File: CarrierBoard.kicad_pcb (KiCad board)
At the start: 2 copper layers, 91.4 x 69.1 mm, 5 parts, among them U5 ESP32-S3-DEVKITC-1U-N8R8

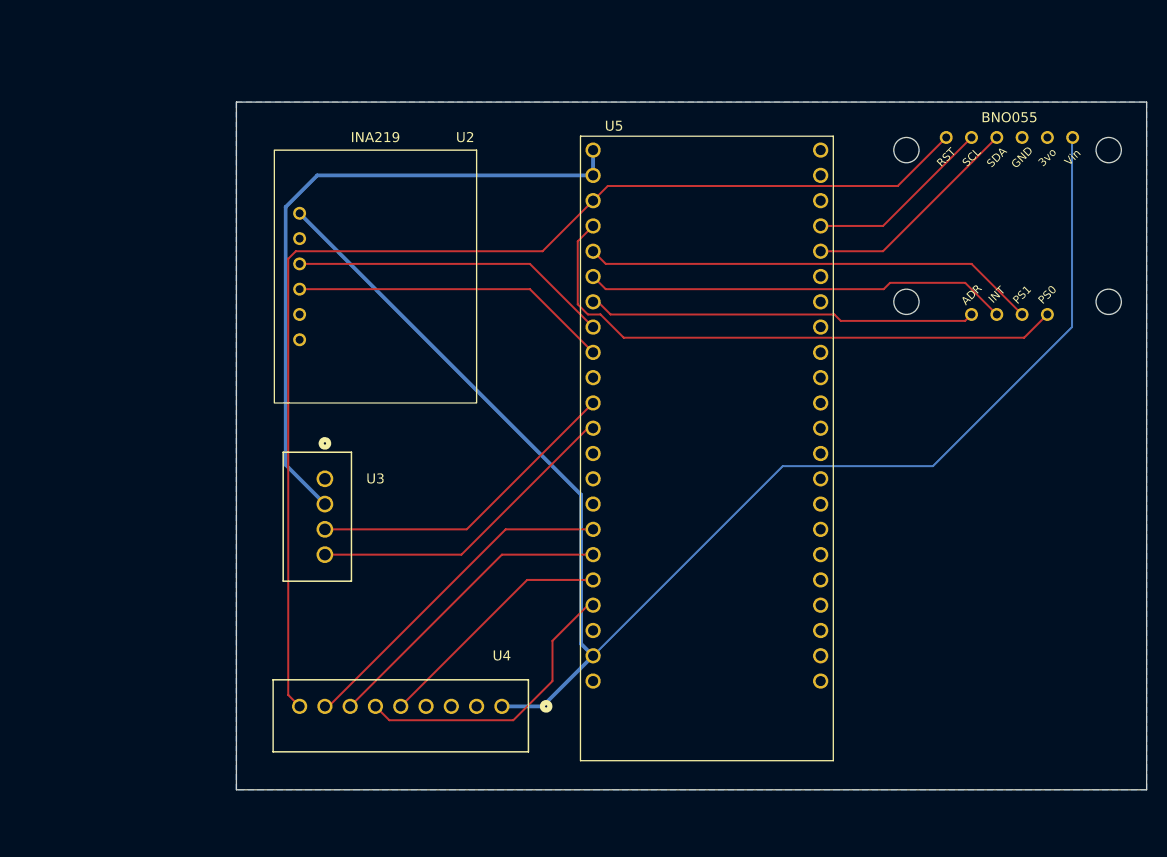
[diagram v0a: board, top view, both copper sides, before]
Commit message: redo board
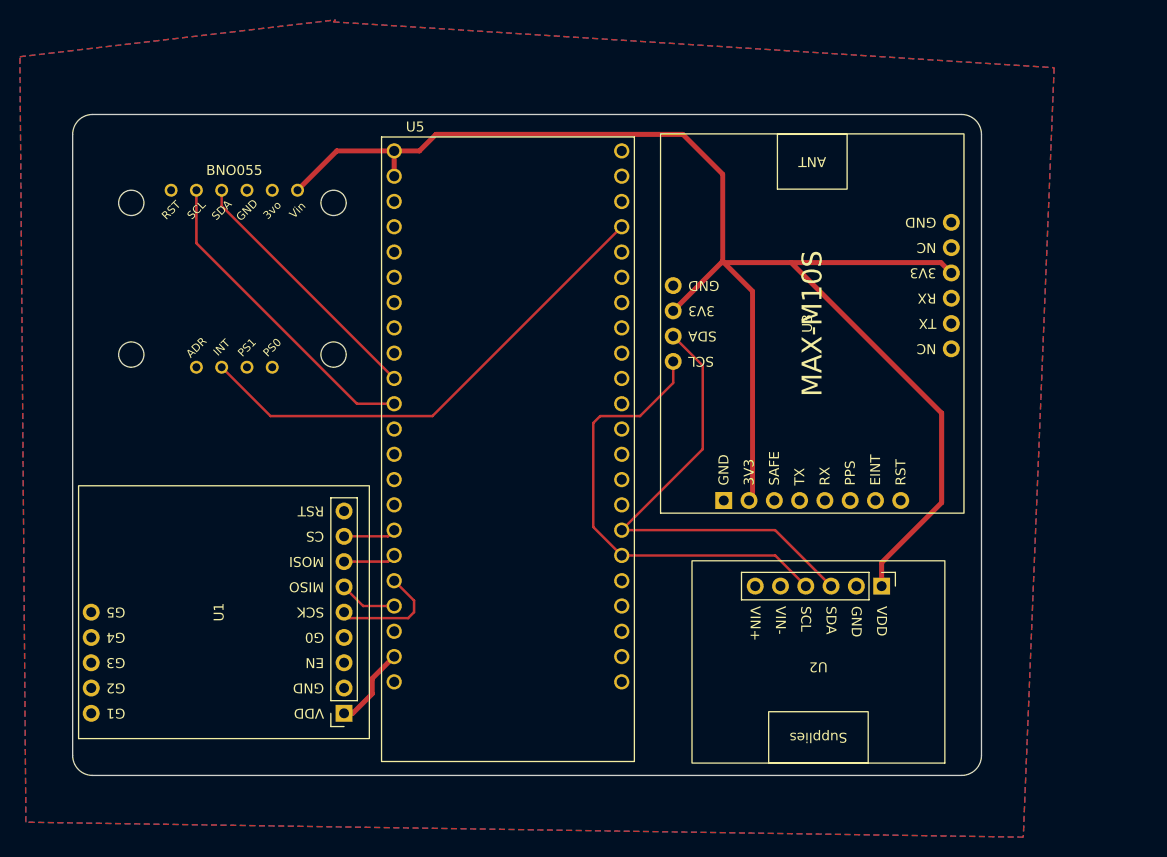
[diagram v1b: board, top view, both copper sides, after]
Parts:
- removed U4: ~, CarrierBoard:TE Connectivity 5-103639-8
- added U6: Adafruit BNO-055, CarrierBoard:Adafruit BNO055, F.Cu at (50.6, 72.6)
- U1: value ~ -> Adafruit RFM95W; footprint CarrierBoard:Adafruit BNO055 -> internalcomponents:Adafruit RFM95W
- U2: value ~ -> Adafruit INA-219; footprint CarrierBoard:Adafruit INA219 -> internalcomponents:INA-219 Adafruit Breakout
- U3: value ~ -> SparkFun MAX-M10S; footprint CarrierBoard:SparkFun MAX-M10S -> internalcomponents:MAX-M10S Sparkfun Breakout
- moved U1 86.8 mm to (55.9, 115.0), turned to 90 degrees
- moved U2 68.9 mm to (115.6, 120.0), turned to 180 degrees
- moved U3 51.4 mm to (115.0, 86.0)
- moved U5 20.0 mm to (84.4, 98.6)
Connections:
- U1 pad 10: Net-(U1-ADR) -> unconnected-(U1-G1-Pad10)
- U1 pad 2: unconnected-(U1-3vo-Pad2) -> GND
- U1 pad 3: GND -> unconnected-(U1-EN-Pad3)
- U1 pad 4: Net-(U1-SDA) -> unconnected-(U1-G0-Pad4)
- U1 pad 5: Net-(U1-SCL) -> /SPI2_SCK
- U1 pad 6: Net-(U1-RST) -> /SPI2_MISO
- U1 pad 7: Net-(U1-PS0) -> /SPI2_MOSI
- U1 pad 8: Net-(U1-PS1) -> /SPI2_CS
- U1 pad 9: Net-(U1-INT) -> unconnected-(U1-RST-Pad9)
- U2 pad 1: +5V -> +3.3V
- U2 pad 3: Net-(U2-SCL) -> /I2C1_SCL
- U2 pad 4: Net-(U2-SDA) -> /I2C1_SDA
- U3 pad 3: Net-(U3-SDA) -> unconnected-(U3-SAFE-Pad3)
- U3 pad 4: Net-(U3-SCL) -> unconnected-(U3-TX-Pad10)
- U5 pad J1_10: unconnected-(U5-GPIO17-PadJ1_10) -> /I2C0_SDA
- U5 pad J1_11: Net-(U3-SDA) -> /I2C0_SCL
- U5 pad J1_12: Net-(U3-SCL) -> unconnected-(U5-GPIO8-PadJ1_12)
- U5 pad J1_16: Net-(U4-CS) -> /SPI2_CS
- U5 pad J1_17: Net-(U4-MOSI) -> /SPI2_MOSI
- U5 pad J1_18: Net-(U4-SCK) -> /SPI2_SCK
- U5 pad J1_19: Net-(U4-MISO) -> /SPI2_MISO
- U5 pad J1_3: Net-(U1-RST) -> unconnected-(U5-RST-PadJ1_3)
- U5 pad J1_4: Net-(U1-PS0) -> unconnected-(U5-GPIO4-PadJ1_4)
- U5 pad J1_5: Net-(U1-PS1) -> unconnected-(U5-GPIO5-PadJ1_5)
- U5 pad J1_6: Net-(U1-INT) -> unconnected-(U5-GPIO6-PadJ1_6)
- U5 pad J1_7: Net-(U1-ADR) -> unconnected-(U5-GPIO7-PadJ1_7)
- U5 pad J1_8: Net-(U2-SCL) -> unconnected-(U5-GPIO15-PadJ1_8)
- U5 pad J1_9: Net-(U2-SDA) -> unconnected-(U5-GPIO16-PadJ1_9)
- U5 pad J3_16: unconnected-(U5-GPIO48-PadJ3_16) -> /I2C1_SCL
- U5 pad J3_17: unconnected-(U5-GPIO47-PadJ3_17) -> /I2C1_SDA
- U5 pad J3_4: Net-(U1-SCL) -> /GYRO_INT
- U5 pad J3_5: Net-(U1-SDA) -> unconnected-(U5-GPIO2-PadJ3_5)
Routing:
- net +5V: track 148.8 -> 8.30 mm
- net Net-(U1-RST): track 116.6 -> 0.00 mm
- net +3.3V: track 66.2 -> 155.2 mm
- net Net-(U1-PS0): track 58.0 -> 0.00 mm
- net /GYRO_INT: track 0.00 -> 50.1 mm
- net /I2C1_SCL: track 0.00 -> 47.4 mm
- net /I2C1_SDA: track 0.00 -> 46.1 mm
- net Net-(U1-PS1): track 45.7 -> 0.00 mm
- net Net-(U1-INT): track 42.7 -> 0.00 mm
- net Net-(U1-ADR): track 39.1 -> 0.00 mm
- net Net-(U4-CS): track 34.3 -> 0.00 mm
- net Net-(U3-SDA): track 32.2 -> 0.00 mm
- net Net-(U3-SCL): track 32.2 -> 0.00 mm
- net Net-(U2-SDA): track 32.1 -> 0.00 mm
- net Net-(U2-SCL): track 32.1 -> 0.00 mm
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- added copper zone on F.Cu, net GND
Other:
- board size 91.4 x 69.1 mm -> 91.3 x 66.4 mm
